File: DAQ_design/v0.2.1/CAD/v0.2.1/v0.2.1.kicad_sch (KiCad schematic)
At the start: 37 parts, among them J1 Screw_Terminal_01x04, U1 Teensy4.0, U2 L293D, U3 PC817, U5 PC817, U6 PC817, U7 74HC165

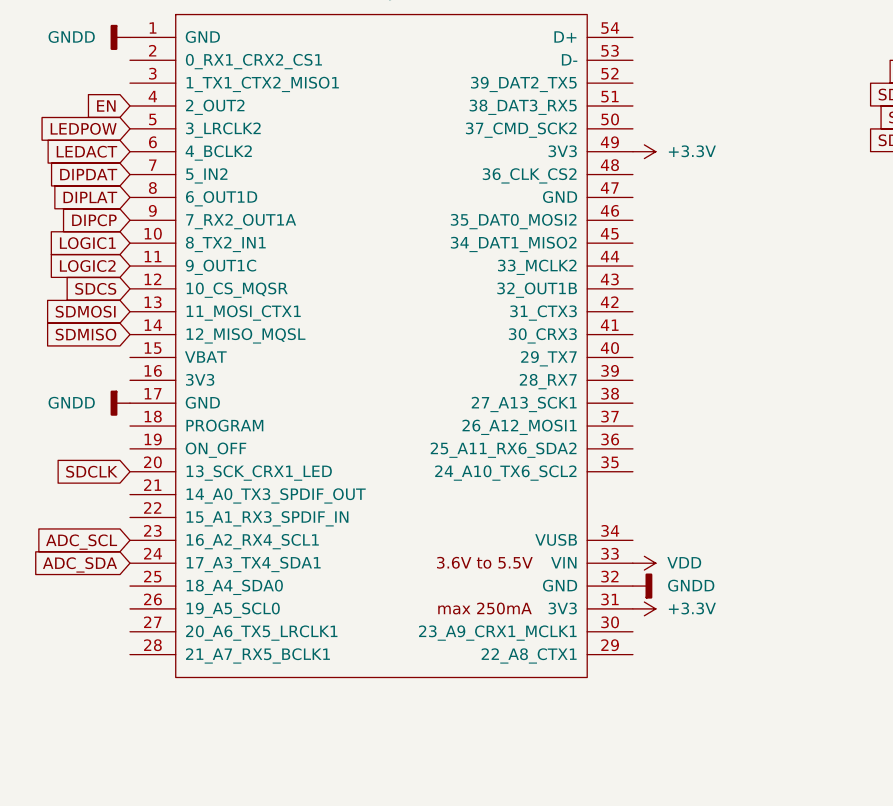
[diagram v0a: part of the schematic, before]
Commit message: v2 trances
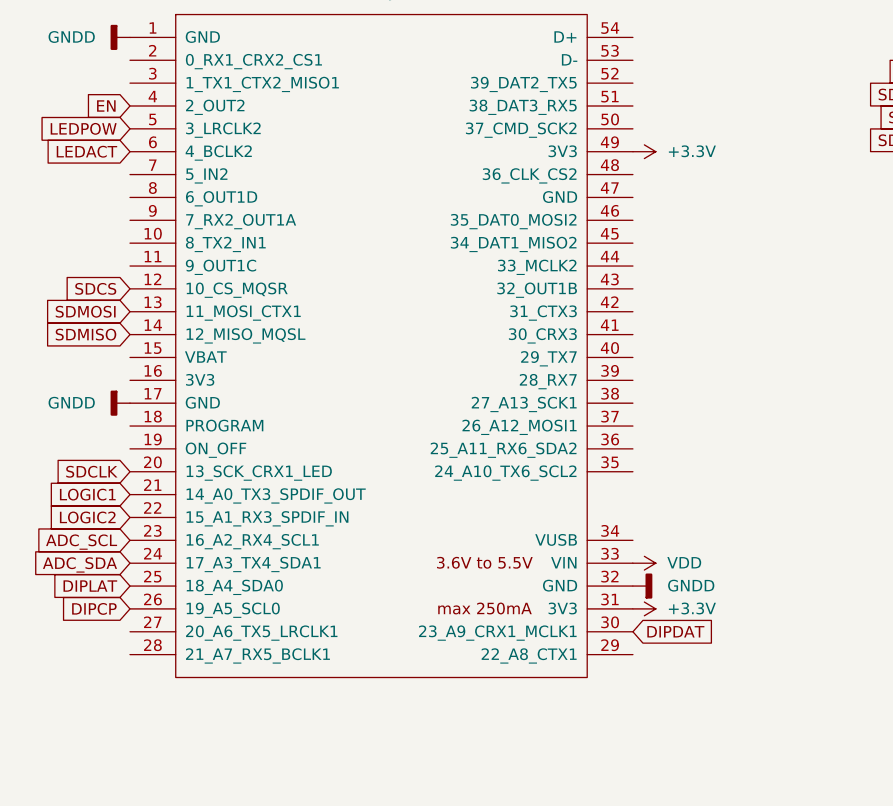
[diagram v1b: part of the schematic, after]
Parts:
- BT1: footprint (none) -> Connector_JST:JST_GH_SM02B-GHS-TB_1x02-1MP_P1.25mm_Horizontal
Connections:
- net DIPCP: now also U1.26 (19_A5_SCL0); no longer U1.9 (7_RX2_OUT1A)
- net DIPDAT: now also U1.30 (23_A9_CRX1_MCLK1); no longer U1.7 (5_IN2)
- net DIPLAT: now also U1.25 (18_A4_SDA0); no longer U1.8 (6_OUT1D)
- net LOGIC1: now also U1.21 (14_A0_TX3_SPDIF_OUT); no longer U1.10 (8_TX2_IN1)
- net LOGIC2: now also U1.22 (15_A1_RX3_SPDIF_IN); no longer U1.11 (9_OUT1C)
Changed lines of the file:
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@@
 		)
 	)
-	(global_label "DIPCP"
-		(shape input)
-		(at 29.21 53.34 180)
-		(fields_autoplaced yes)
-		(effects
-			(font
-				(size 1.27 1.27)
-			)
-			(justify right)
-		)
-		(property "Intersheetrefs" "${INTERSHEET_REFS}"
-			(at 20.54 53.34 0)
-			(effects
-				(font
-					(size 1.27 1.27)
-				)
-				(justify right)
-				(hide yes)
-			)
-		)
-	)
-	(global_label "DIPLAT"
-		(shape input)
-		(at 29.21 50.8 180)
-		(fields_autoplaced yes)
-		(effects
-			(font
-				(size 1.27 1.27)
-			)
-			(justify right)
-		)
-		(property "Intersheetrefs" "${INTERSHEET_REFS}"
-			(at 19.9957 50.8 0)
-			(effects
-				(font
-					(size 1.27 1.27)
-				)
-				(justify right)
-				(hide yes)
-			)
-		)
-	)
 	(global_label "IN0"
 		(shape input)
@@
 		)
 	)
-	(global_label "DIPDAT"
-		(shape input)
-		(at 29.21 48.26 180)
-		(fields_autoplaced yes)
-		(effects
-			(font
-				(size 1.27 1.27)
-			)
-			(justify right)
-		)
-		(property "Intersheetrefs" "${INTERSHEET_REFS}"
-			(at 19.7538 48.26 0)
-			(effects
-				(font
-					(size 1.27 1.27)
-				)
-				(justify right)
-				(hide yes)
-			)
-		)
-	)
 	(global_label "DIPCP"
 		(shape input)
@@
 	(global_label "LOGIC1"
 		(shape input)
-		(at 29.21 55.88 180)
+		(at 29.21 83.82 180)
 		(fields_autoplaced yes)
 		(effects
@@
 		)
 		(property "Intersheetrefs" "${INTERSHEET_REFS}"
-			(at 19.5119 55.88 0)
+			(at 19.5119 83.82 0)
 			(effects
 				(font
@@
 		)
 	)
+	(global_label "DIPCP"
+		(shape input)
+		(at 29.21 96.52 180)
+		(fields_autoplaced yes)
+		(effects
+			(font
+				(size 1.27 1.27)
+			)
+			(justify right)
+		)
+		(property "Intersheetrefs" "${INTERSHEET_REFS}"
+			(at 20.54 96.52 0)
+			(effects
+				(font
+					(size 1.27 1.27)
+				)
+				(justify right)
+				(hide yes)
+			)
+		)
+	)
 	(global_label "SDCLK"
 		(shape input)
@@
 	(global_label "LOGIC2"
 		(shape input)
-		(at 29.21 58.42 180)
+		(at 29.21 86.36 180)
 		(fields_autoplaced yes)
 		(effects
@@
 		)
 		(property "Intersheetrefs" "${INTERSHEET_REFS}"
-			(at 19.5119 58.42 0)
+			(at 19.5119 86.36 0)
 			(effects
 				(font
@@
 		)
 	)
+	(global_label "DIPLAT"
+		(shape input)
+		(at 29.21 93.98 180)
+		(fields_autoplaced yes)
+		(effects
+			(font
+				(size 1.27 1.27)
+			)
+			(justify right)
+		)
+		(property "Intersheetrefs" "${INTERSHEET_REFS}"
+			(at 19.9957 93.98 0)
+			(effects
+				(font
+					(size 1.27 1.27)
+				)
+				(justify right)
+				(hide yes)
+			)
+		)
+	)
 	(global_label "SDCS"
 		(shape input)
@@
 		)
 	)
+	(global_label "DIPDAT"
+		(shape input)
+		(at 85.09 99.06 0)
+		(fields_autoplaced yes)
+		(effects
+			(font
+				(size 1.27 1.27)
+			)
+			(justify left)
+		)
+		(property "Intersheetrefs" "${INTERSHEET_REFS}"
+			(at 94.5462 99.06 0)
+			(effects
+				(font
+					(size 1.27 1.27)
+				)
+				(justify left)
+				(hide yes)
+			)
+		)
+	)
 	(global_label "SW7"
 		(shape input)
@@
 			)
 		)
-		(property "Footprint" ""
+		(property "Footprint" "Connector_JST:JST_GH_SM02B-GHS-TB_1x02-1MP_P1.25mm_Horizontal"
 			(at 196.85 149.606 90)
 			(effects
